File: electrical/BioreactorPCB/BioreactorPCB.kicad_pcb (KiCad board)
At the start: 2 copper layers, 68 parts, among them IC1 AL5809-20P1-7, IC2 VEML7700-TR, J1 61300311121, J10 USB_B, J11 Conn_01x06_Male, J12 Conn_02x03_Odd_Even, J13 PJ-202A, J14 Conn_01x05_Male, J2 61300311121, J3 Conn_01x05_Male, J4 Conn_01x06_Male, J5 OSTTC022162, J6 OSTTC022162, J7 OSTTC042162, J8 OSTTC042162, J9 OSTTC042162, Q1 2N3905, Q2 IRF540N, Q3 FQP47P06, Q4 TL2575HV-05IKV, U1 L293D, U2 FT232RL, U3 ATMEGA328P-AUR, U4 TCA39306DCUR, Y1 16 mHz

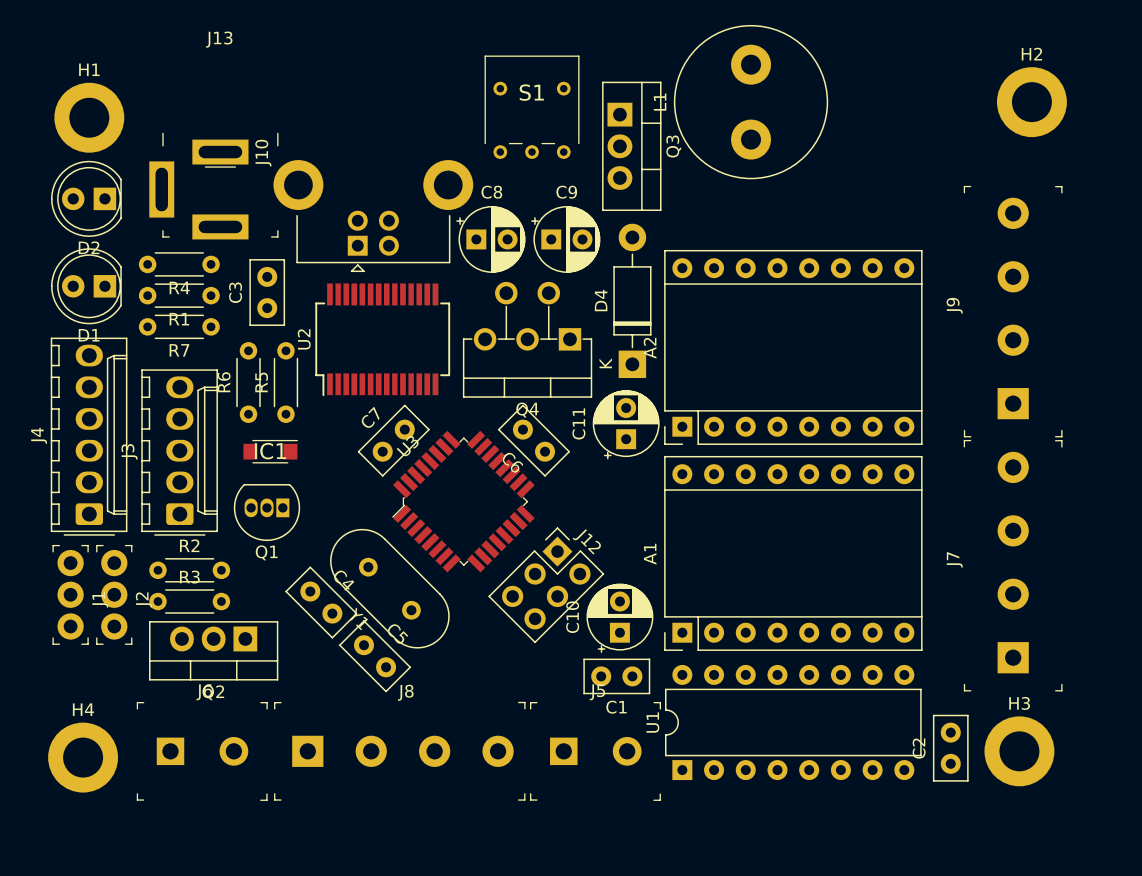
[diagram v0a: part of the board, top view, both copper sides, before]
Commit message: motherboard layout complete.
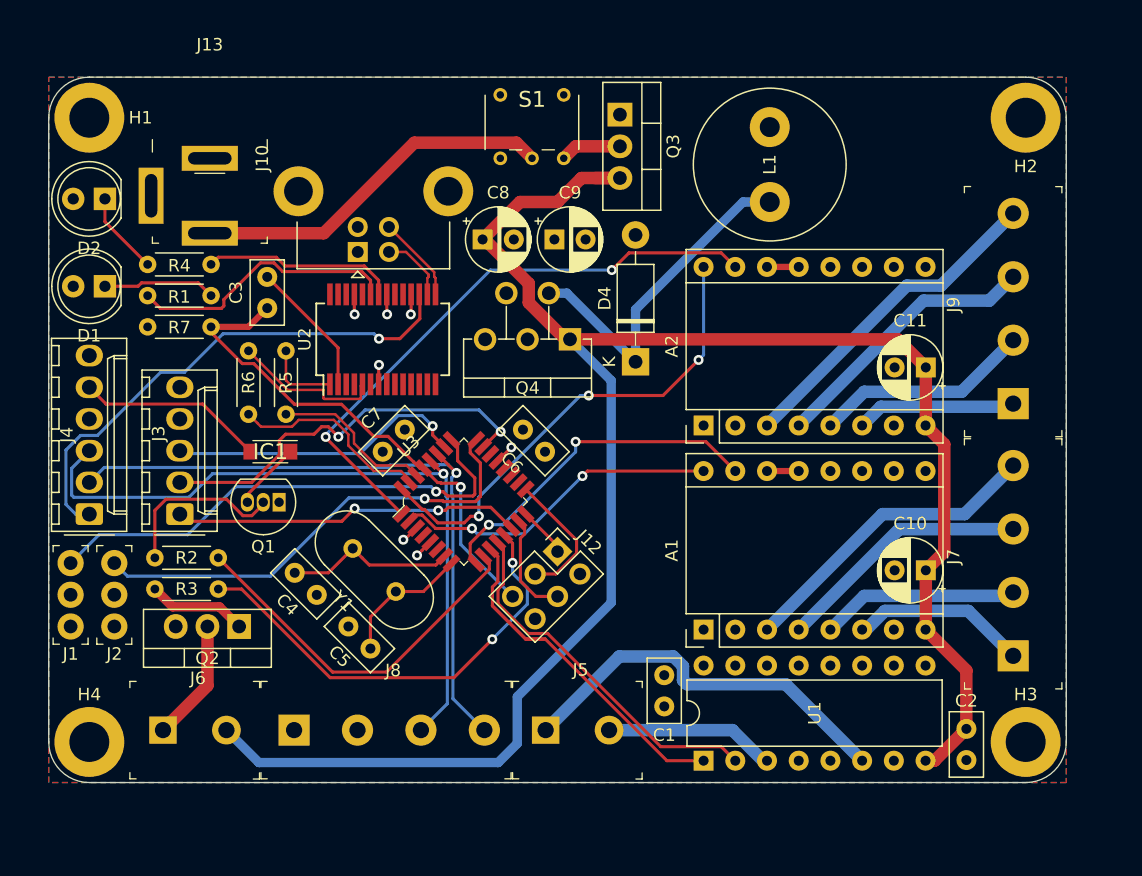
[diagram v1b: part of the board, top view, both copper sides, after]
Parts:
- moved C10 25.0 mm to (152.0, 77.0), turned to 180 degrees
- moved C11 24.7 mm to (152.0, 60.8), turned to 180 degrees
- moved L1 5.22 mm to (139.5, 47.5)
- moved C1 2.55 mm to (131.1, 85.4), turned to 270 degrees
- moved J5 2.23 mm to (121.5, 89.8)
- moved J8 2.02 mm to (101.4, 89.8)
- moved C4 1.95 mm to (101.5, 77.2)
- moved C5 1.95 mm to (105.8, 81.5)
- moved Y1 1.95 mm to (109.5, 78.7)
- moved U1 1.86 mm to (134.2, 92.2)
- moved J6 1.80 mm to (90.9, 89.8)
- moved A1 1.72 mm to (134.2, 81.8)
- moved A2 1.70 mm to (134.2, 65.4)
- moved H2 1.35 mm to (160.0, 40.8)
- moved H4 1.35 mm to (85.0, 90.8)
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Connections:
- net Net-(C4-Pad1) renamed XTAL+
- net Net-(C5-Pad2) renamed XTAL-
- net Net-(J10-Pad2) renamed D-
- net Net-(J10-Pad3) renamed D+
- net Net-(R5-Pad1) renamed RX_TX_P
- net Net-(R6-Pad1) renamed RX_TX_N
- net RX renamed RX_TX_+
- net TX renamed RX_TX_-
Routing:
- net +12V: track 0.00 -> 153.4 mm
- net SCL: track 0.00 -> 57.8 mm, vias 0 -> 1
- net SDA: track 0.00 -> 54.3 mm, vias 0 -> 1
- net D3: track 0.00 -> 48.6 mm, vias 0 -> 2
- net +3V3: track 0.00 -> 41.5 mm, vias 0 -> 1
- net RESET: track 0.00 -> 41.2 mm, vias 0 -> 1
- net TEMP_OUT: track 0.00 -> 40.4 mm, vias 0 -> 1
- net D2: track 0.00 -> 38.8 mm, vias 0 -> 3
- net PH_OUT: track 0.00 -> 37.7 mm, vias 0 -> 1
- net D9: track 0.00 -> 36.4 mm, vias 0 -> 2
- net D7: track 0.00 -> 33.1 mm
- net ROT_A: track 0.00 -> 32.1 mm, vias 0 -> 2
- net Net-(J5-Pad1): track 0.00 -> 31.9 mm
- net D6: track 0.00 -> 30.1 mm
- net D8: track 0.00 -> 29.5 mm
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- added copper zone on F.Cu, net +5V
- added copper zone on B.Cu, net GND
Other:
- board outline added: 81.5 x 56.5 mm
